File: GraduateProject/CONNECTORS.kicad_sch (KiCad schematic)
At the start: 62 parts, among them J2 Conn_01x05_Pin, J3 Conn_01x05_Pin, J4 Conn_01x04_Pin, J6 Conn_01x04_Pin, Q10 IMX1T110, Q11 IMX1T110, Q12 IMX1T110, Q2 BST50,115, Q3 IMX1T110, Q4 IMX1T110, Q5 IMT2AT108, Q6 IMT2AT108, Q7 IMX1T110, Q8 IMX1T110, Q9 IMX1T110

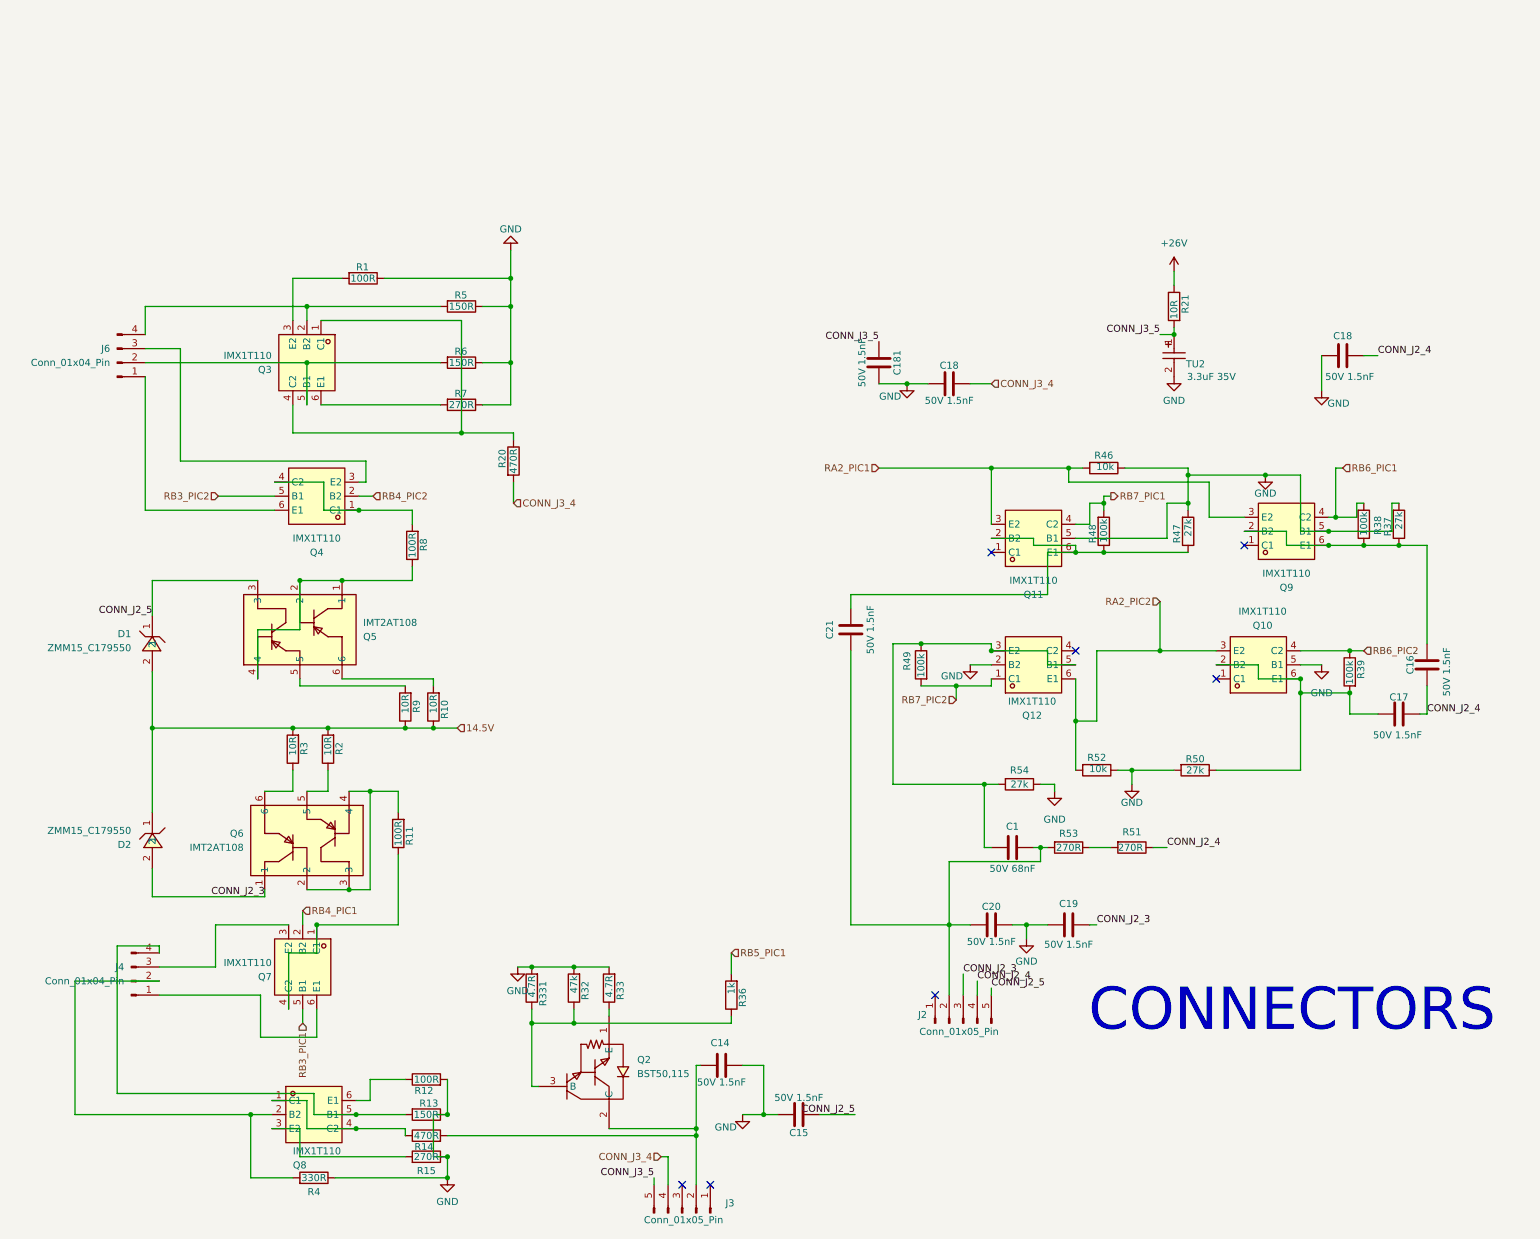
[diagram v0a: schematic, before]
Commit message: Add files via upload
10/9/25
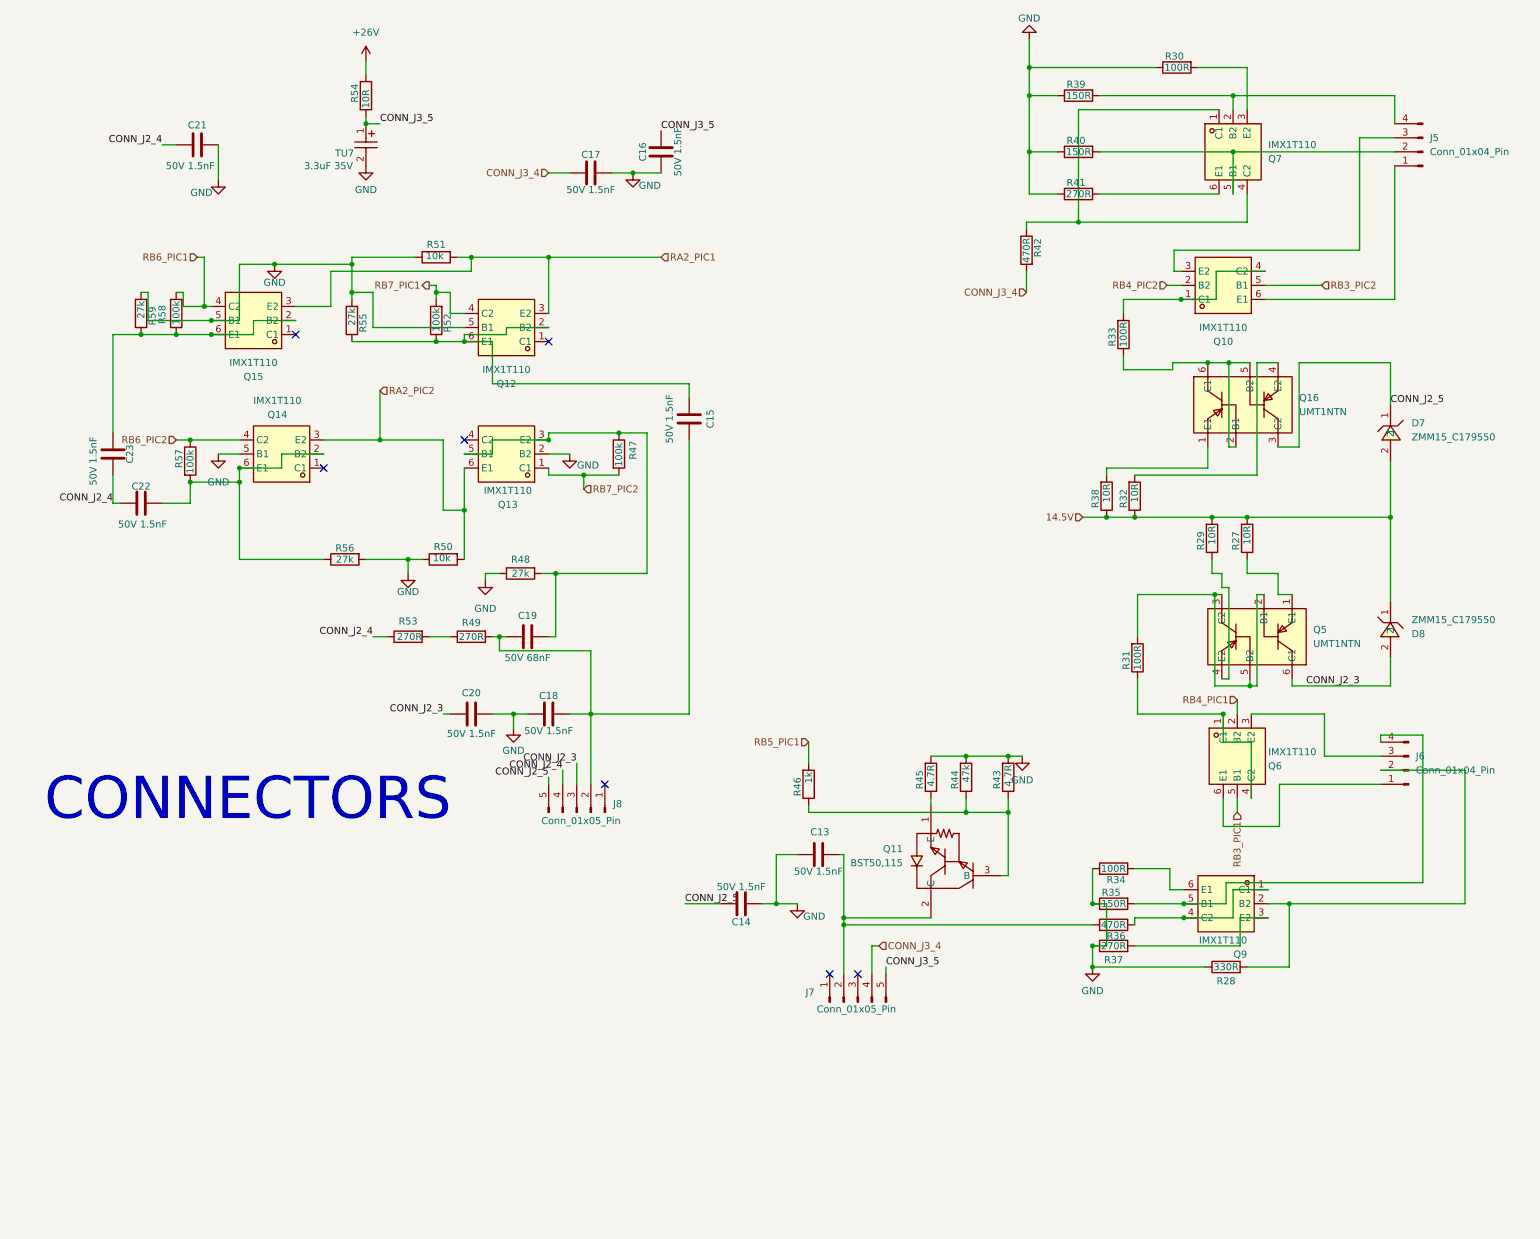
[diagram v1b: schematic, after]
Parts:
- removed Q5, Q6: IMT2AT108, easyeda2kicad:SOT-457-6_L2.9-W1.7-P0.95-LS2.8-BR, symbol easyeda2kicad:IMT2AT108
- added Q16, Q5: UMT1NTN, easyeda2kicad:SC-70-6_L2.2-W1.3-P0.65-LS2.1-TL, symbol easyeda2kicad:UMT1NTN
- J5: renamed from J6; footprint (none) -> Connector_PinHeader_2.54mm:PinHeader_1x04_P2.54mm_Vertical
- J6: renamed from J4; footprint (none) -> Connector_PinHeader_2.54mm:PinHeader_1x04_P2.54mm_Vertical
- J7: renamed from J3; footprint (none) -> Connector_PinHeader_2.54mm:PinHeader_1x05_P2.54mm_Vertical
- J8: renamed from J2; footprint (none) -> Connector_PinHeader_2.54mm:PinHeader_1x05_P2.54mm_Vertical
- renumbered C14 to C13, C15 to C14, C21 to C15, C181 to C16, C18 to C17, C20 to C18, C1 to C19, C19 to C20, C18 to C21, C17 to C22, C16 to C23, D1 to D7, D2 to D8, Q4 to Q10, Q2 to Q11, Q11 to Q12, Q12 to Q13, Q10 to Q14, Q9 to Q15, Q7 to Q6, Q3 to Q7, Q8 to Q9, R3 to R27, R4 to R28, R2 to R29, R1 to R30, R11 to R31, R9 to R32, R8 to R33, R12 to R34, R13 to R35, R14 to R36, R15 to R37, R10 to R38, R5 to R39, R6 to R40, R7 to R41, R20 to R42, R331 to R43, R32 to R44, R33 to R45, R36 to R46, R49 to R47, R54 to R48, R53 to R49, R52 to R50, R46 to R51, R48 to R52, R51 to R53, R21 to R54, R47 to R55, R50 to R56, R39 to R57, R38 to R58, R37 to R59, TU2 to TU7
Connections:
- net CONN_J2_3: now also Q5.6 (C1)
- net CONN_J2_5: now also Q16.3 (C2)
- net at R27.1: now also Q5.1 (E1)
- net at R31.2: now also Q5.2 (B1), Q5.3 (C2), Q5.5 (B2)
- net at R29.1: now also Q5.4 (E2)
- net at R33.1: now also Q16.2 (B1), Q16.5 (B2), Q16.6 (C1)
- net at R32.2: now also Q16.4 (E2)
- net at R38.2: now also Q16.1 (E1)
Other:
- moved on the sheet: C13, C14, C15, C16, C17, C18, C19, C20, C21, C22, C23, D7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
